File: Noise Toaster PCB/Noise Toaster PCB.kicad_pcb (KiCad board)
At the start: 2 copper layers, 170 x 97.5 mm, 133 parts, among them Q1 2N5457, Q10 2N3906, Q2 2N3904, Q3 2N3904, Q4 2N3904, Q5 2N3904, Q6 2N3904, Q7 2N5457, Q8 2N5457, Q9 2N5457, U1 LM324, U2 LM324, U3 LM386, X10 Conn_01x01_Pin, X11 Conn_01x01_Pin, X12 Conn_01x01_Pin, X13 Conn_01x01_Pin, X14 Conn_01x01_Pin, X24 Conn_01x01_Pin, X25 Conn_01x01_Pin, X26 Conn_01x01_Pin, X27 Conn_01x01_Pin, X8 Conn_01x01_Pin, X9 Conn_01x01_Pin

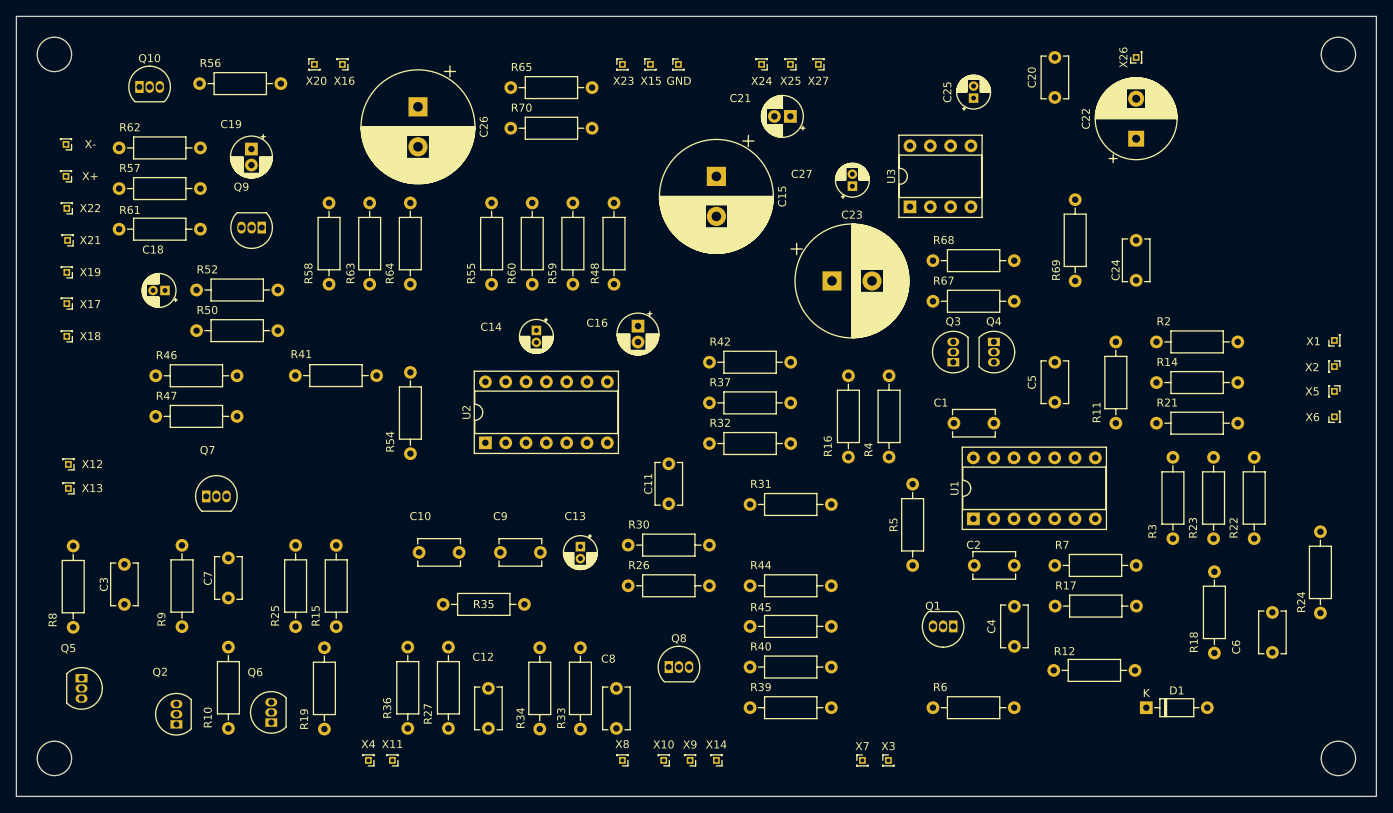
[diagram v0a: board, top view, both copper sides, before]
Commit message: created pcb file
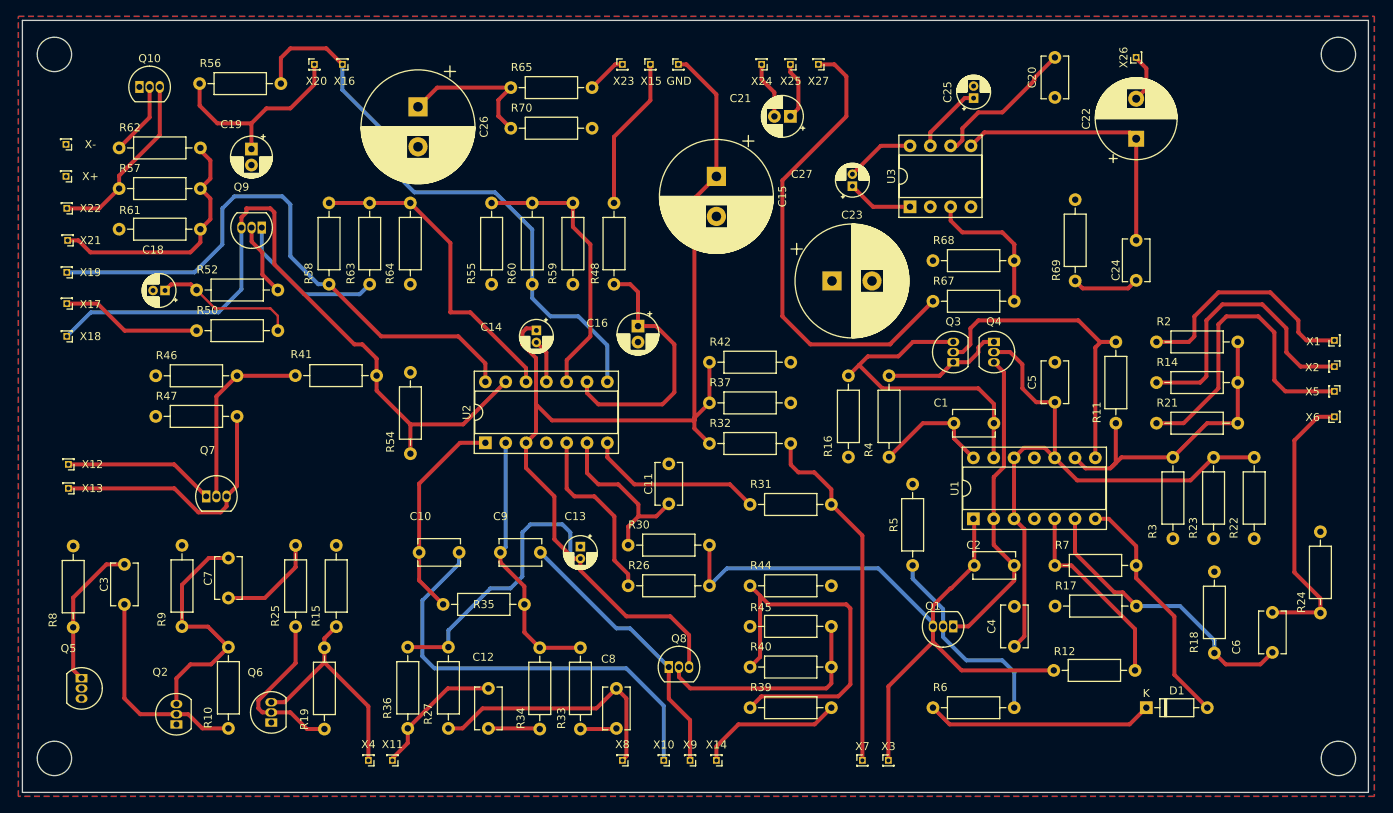
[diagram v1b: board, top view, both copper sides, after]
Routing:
- net GND: track 0.00 -> 173.6 mm
- net /ARG: track 0.00 -> 90.3 mm
- net /RMP: track 0.00 -> 88.5 mm
- net /G2: track 0.00 -> 77.0 mm
- net /Attack Release Envelope Generator/X19: track 0.00 -> 73.7 mm
- net /Front Panel/B: track 0.00 -> 73.6 mm
- net /Audio Amplifier/X27: track 0.00 -> 60.0 mm
- net /Front Panel/X10: track 0.00 -> 54.5 mm
- net Net-(R39-Pad2): track 0.00 -> 46.4 mm
- net /SQR: track 0.00 -> 44.5 mm
- net Net-(Q3-C): track 0.00 -> 40.5 mm
- net Net-(U2D-+): track 0.00 -> 40.0 mm
- net /Front Panel/X5: track 0.00 -> 39.9 mm
- net /AA: track 0.00 -> 39.4 mm
- net Net-(Q3-B): track 0.00 -> 39.0 mm
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- added copper zone on F.Cu, net B+
- added copper zone on B.Cu, net B-
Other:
- board size 170 x 97.5 mm -> 168.2 x 96.5 mm
